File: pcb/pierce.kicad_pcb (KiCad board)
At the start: 2 copper layers, 227.3 x 105.6 mm, 100 parts, among them J1 Conn_01x12, J2 Conn_01x12, J3 Trackpoint, SW1 SW_PUSH, SW10 SW_PUSH, SW11 SW_PUSH, SW12 SW_PUSH, SW13 SW_PUSH, SW14 SW_PUSH, SW15 SW_PUSH, SW16 SW_PUSH, SW17 SW_PUSH, SW18 SW_PUSH, SW19 SW_PUSH, SW2 SW_PUSH, SW20 SW_PUSH, SW21 SW_PUSH, SW22 SW_PUSH, SW23 SW_PUSH, SW24 SW_PUSH, SW25 SW_PUSH, SW26 SW_PUSH, SW27 SW_PUSH, SW28 SW_PUSH, SW29 SW_PUSH, SW3 SW_PUSH, SW30 SW_PUSH, SW31 SW_PUSH, SW32 SW_PUSH, SW33 SW_PUSH, SW34 SW_PUSH, SW35 SW_PUSH, SW36 SW_PUSH, SW37 SW_PUSH, SW38 Rotary_Encoder, SW4 SW_PUSH, SW5 SW_PUSH, SW6 SW_PUSH, SW7 SW_PUSH, SW8 SW_PUSH, SW9 SW_PUSH, U1 Elite-C_reverse

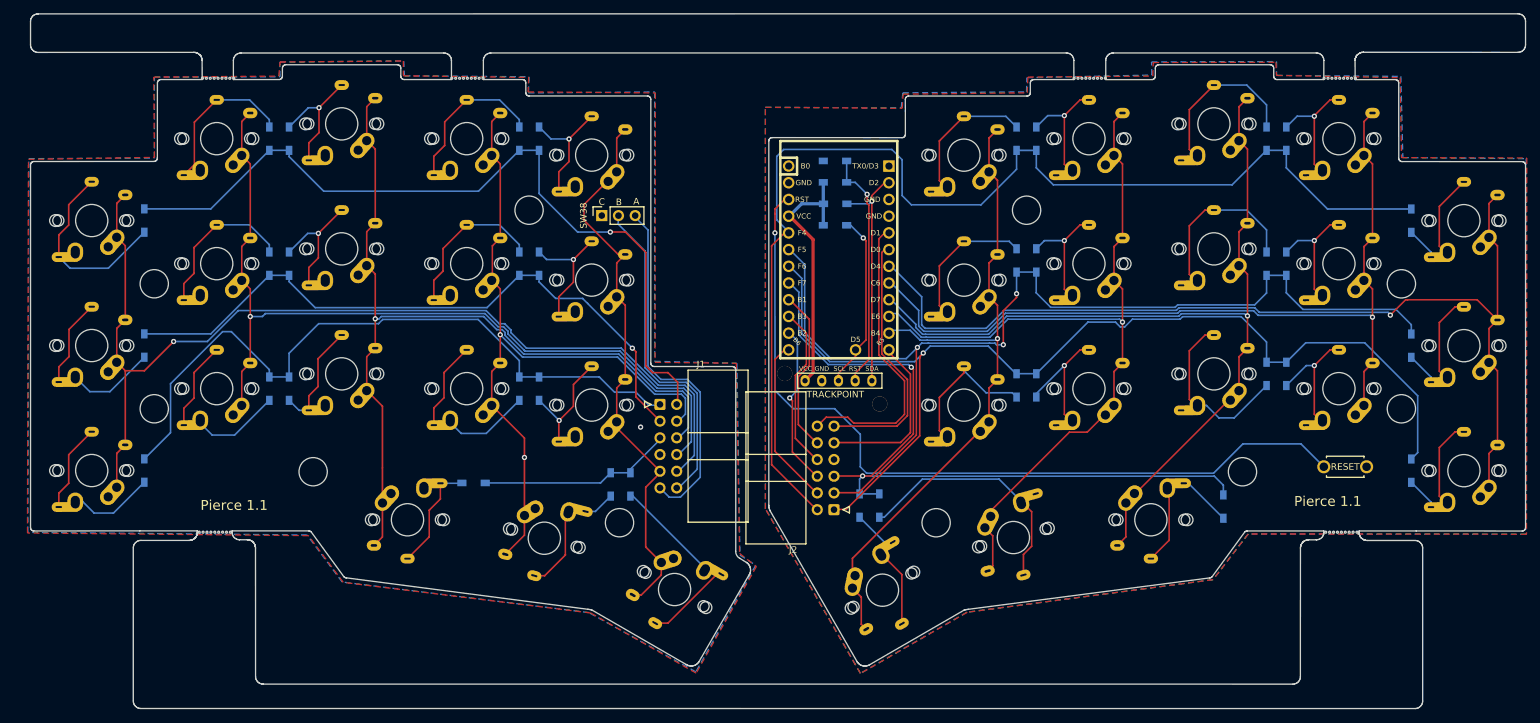
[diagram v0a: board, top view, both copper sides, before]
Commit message: place and route 2.0
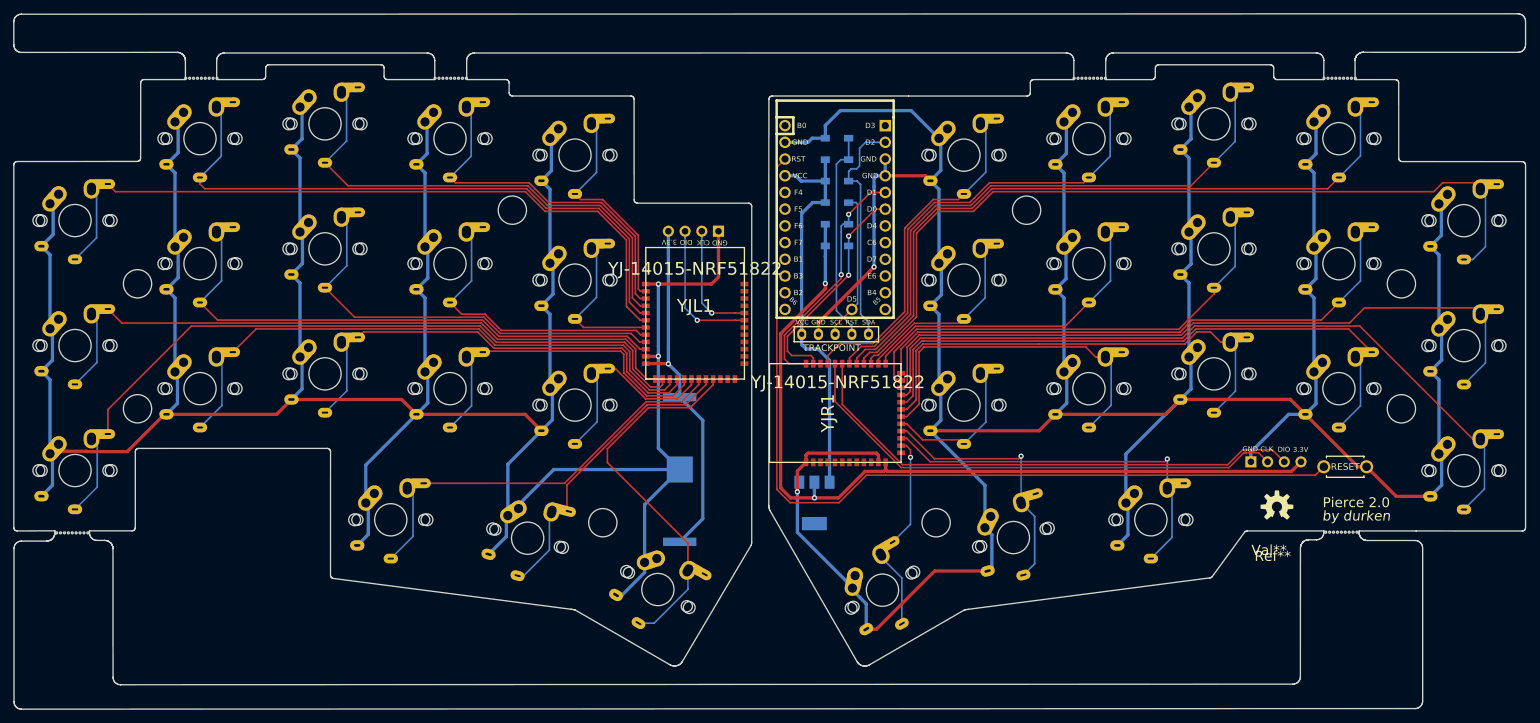
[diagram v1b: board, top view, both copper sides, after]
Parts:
- removed D1, D10, D11, D12, D13, D14, D15, D16, D17, D18, D19, D2, D20, D21, D22, D23, D24, D25, D26, D27, D28, D29, D3, D30, D31, D32, D33, D34, D35, D36, D4, D5, D6, D7, D8, D9: D, kbd:D3_SMD_v2
- removed J1, J2: Conn_01x12, Connector_IDC:IDC-Header_2x06_P2.54mm_Horizontal
- removed J3: Trackpoint, pierce:TRACKPOINT
- removed the REF** at (62.9, 95.0)
- removed the REF** at (101.3, 26.0)
- removed the REF** at (63.4, 26.0)
- removed the Ref** at (53.7, 57.3)
- removed the Ref** at (219.1, 85.8)
- removed the Ref** at (149.5, 70.9)
- removed the Ref** at (162.6, 75.5)
- removed the Ref** at (53.7, 76.3)
- removed the Ref** at (110.6, 46.1)
- removed the Ref** at (124.4, 93.6)
- removed the Ref** at (77.8, 85.8)
- removed SW38: Rotary_Encoder, pierce:Rotary_encoder_conn
- added BT1: Device_Battery_Cell, pierce:BatteryHolder_Keystone_3034_1x20mm, B.Cu at (133.6, 85.5)
- added PROGL1: Conn_01x04_Male, pierce:PinHeader_1x04_P2.54mm_Horizontal, B.Cu at (139.4, 49.3)
- added PROGR1: Conn_01x04_Male, pierce:PinHeader_1x04_P2.54mm_Horizontal, B.Cu at (220.4, 84.3)
- added R4: 4k7, pierce:R_SMD_v2, B.Cu at (157.5, 51.5)
- added R5: 4k7, pierce:R_SMD_v2, B.Cu at (157.5, 48.2)
- added REF**: Breakaway_Tabs, kbd:Breakaway_Tabs, F.Cu at (41.2, 95.1)
- added REF**: Breakaway_Tabs, kbd:Breakaway_Tabs, F.Cu at (98.7, 26.0)
- added REF**: Breakaway_Tabs, kbd:Breakaway_Tabs, F.Cu at (60.8, 26.0)
- added REG1: LD1117S33TR_SOT223, Package_TO_SOT_SMD:SOT-223-3_TabPin2, B.Cu at (154.0, 90.6)
- added Ref**: Val**, pierce:OSHW-LOGO-M, B.Cu at (224.3, 91.2)
- added Ref**: Val**, pierce:OSHW-LOGO-M, F.Cu at (224.3, 91.2)
- added Ref**: Val**, kbd:M2_HOLE_v2, F.Cu at (51.1, 57.3)
- added Ref**: Val**, kbd:M2_HOLE_v2, F.Cu at (51.1, 76.3)
- added Ref**: Val**, kbd:M2_HOLE_v2, F.Cu at (108.1, 46.1)
- added Ref**: Val**, kbd:M2_HOLE_v2, F.Cu at (121.9, 93.6)
- added TP1: Trackpoint, pierce:TRACKPOINT, F.Cu at (152.1, 64.9)
- added YJL1: YJ-14015-NRF51822, pierce:YJ-14015, F.Cu at (135.9, 71.8)
- added YJR1: YJ-14015-NRF51822, pierce:YJ-14015, F.Cu at (167.2, 76.9)
- SW1, SW10, SW11, SW12, SW13, SW14, SW15, SW16, SW17, SW18, SW19, SW2, SW20, SW21, SW22, SW23, SW24, SW25, SW26, SW27, SW28, SW29, SW3, SW30, SW31, SW32, SW33, SW34, SW35, SW36, SW4, SW5, SW6, SW7, SW8, SW9: footprint kbd:keyswitch_cherrymx_alps_choc12_1u -> pierce:keyswitch_cherrymx_alps_choc12_1u
- moved AVR1 6.17 mm to (156.9, 47.2)
- moved R1 3.47 mm to (157.5, 35.1)
- moved C1 3.47 mm to (157.5, 38.4)
- moved R2 3.47 mm to (157.5, 44.9)
- moved R3 3.47 mm to (157.5, 41.7)
- moved SW33 2.54 mm to (130.2, 103.7)
- moved SW15 2.54 mm to (79.6, 33.0), turned to 0 degrees
- moved SW16 2.54 mm to (79.6, 52.0), turned to 0 degrees
- moved SW17 2.54 mm to (79.6, 71.0), turned to 0 degrees
- moved SW18 2.54 mm to (89.6, 93.1)
- moved SW23 2.54 mm to (98.6, 35.2), turned to 0 degrees
- moved SW24 2.54 mm to (98.6, 54.2), turned to 0 degrees
- moved SW25 2.54 mm to (98.6, 73.2), turned to 0 degrees
- moved SW30 2.54 mm to (117.6, 37.7), turned to 0 degrees
- moved SW31 2.54 mm to (117.6, 56.7), turned to 0 degrees
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- renumbered U1 to AVR1, SW37 to RST1
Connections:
- net VCC renamed VCC_R_5V
- AVR1 pad 10: col6 -> Net-(AVR1-Pad10)
- AVR1 pad 11: col5 -> Net-(AVR1-Pad11)
- AVR1 pad 12: col4 -> Net-(AVR1-Pad12)
- AVR1 pad 13: col3 -> Net-(AVR1-Pad13)
- AVR1 pad 14: col2 -> Net-(AVR1-Pad14)
- AVR1 pad 15: col1 -> Net-(AVR1-Pad15)
- AVR1 pad 16: col0 -> Net-(AVR1-Pad16)
- AVR1 pad 17: row3 -> Net-(AVR1-Pad17)
- AVR1 pad 18: row2 -> Net-(AVR1-Pad18)
- AVR1 pad 19: row1 -> Net-(AVR1-Pad19)
- AVR1 pad 20: row0 -> Net-(AVR1-Pad20)
- AVR1 pad 23: GND -> GND_R
- AVR1 pad 3: GND -> GND_R
- AVR1 pad 4: GND -> GND_R
- AVR1 pad 5: rotb -> I2C_SDA
- AVR1 pad 6: rota -> I2C_SCL
- AVR1 pad 7: col9 -> Net-(AVR1-Pad7)
- AVR1 pad 8: col8 -> Net-(AVR1-Pad8)
- AVR1 pad 9: col7 -> Net-(AVR1-Pad9)
- R1 pad 1: GND -> GND_R
- RST1 pad 2: GND -> GND_R
- SW1 pad 1: col0l -> GND_L
- SW1 pad 2: Net-(D1-Pad2) -> SW00L
- SW10 pad 1: col1l -> GND_L
- SW10 pad 2: Net-(D10-Pad2) -> SW21L
- SW11 pad 1: col6 -> GND_R
- SW11 pad 2: Net-(D11-Pad2) -> SW01R
- SW12 pad 1: col6 -> GND_R
- SW12 pad 2: Net-(D12-Pad2) -> SW11R
- SW13 pad 1: col6 -> GND_R
- SW13 pad 2: Net-(D13-Pad2) -> SW21R
- SW14 pad 1: col6 -> GND_R
- SW14 pad 2: Net-(D14-Pad2) -> SW31R
- SW15 pad 1: col2l -> GND_L
- SW15 pad 2: Net-(D15-Pad2) -> SW02L
- SW16 pad 1: col2l -> GND_L
- SW16 pad 2: Net-(D16-Pad2) -> SW12L
- SW17 pad 1: col2l -> GND_L
- SW17 pad 2: Net-(D17-Pad2) -> SW22L
- SW18 pad 1: col2l -> GND_L
- SW18 pad 2: Net-(D18-Pad2) -> SW32L
- SW19 pad 1: col7 -> GND_R
- SW19 pad 2: Net-(D19-Pad2) -> SW02R
- SW2 pad 1: col0l -> GND_L
- SW2 pad 2: Net-(D2-Pad2) -> SW10L
- SW20 pad 1: col7 -> GND_R
- SW20 pad 2: Net-(D20-Pad2) -> SW12R
- SW21 pad 1: col7 -> GND_R
- SW21 pad 2: Net-(D21-Pad2) -> SW22R
- SW22 pad 1: col7 -> GND_R
- SW22 pad 2: Net-(D22-Pad2) -> SW32R
- SW23 pad 1: col3l -> GND_L
- SW23 pad 2: Net-(D23-Pad2) -> SW03L
- SW24 pad 1: col3l -> GND_L
- SW24 pad 2: Net-(D24-Pad2) -> SW13L
- SW25 pad 1: col3l -> GND_L
- SW25 pad 2: Net-(D25-Pad2) -> SW23L
- SW26 pad 1: col3l -> GND_L
- SW26 pad 2: Net-(D26-Pad2) -> SW33L
- SW27 pad 1: col8 -> GND_R
- SW27 pad 2: Net-(D27-Pad2) -> SW03R
- SW28 pad 1: col8 -> GND_R
- SW28 pad 2: Net-(D28-Pad2) -> SW13R
- SW29 pad 1: col8 -> GND_R
- SW29 pad 2: Net-(D29-Pad2) -> SW23R
- SW3 pad 1: col0l -> GND_L
- SW3 pad 2: Net-(D3-Pad2) -> SW20L
- SW30 pad 1: col4l -> GND_L
- SW30 pad 2: Net-(D30-Pad2) -> SW04L
- SW31 pad 1: col4l -> GND_L
- SW31 pad 2: Net-(D31-Pad2) -> SW14L
- SW32 pad 1: col4l -> GND_L
- SW32 pad 2: Net-(D32-Pad2) -> SW24L
- SW33 pad 1: col4l -> GND_L
- SW33 pad 2: Net-(D33-Pad2) -> SW34L
- SW34 pad 1: col9 -> GND_R
- SW34 pad 2: Net-(D34-Pad2) -> SW04R
- SW35 pad 1: col9 -> GND_R
- SW35 pad 2: Net-(D35-Pad2) -> SW14R
- SW36 pad 1: col9 -> GND_R
- SW36 pad 2: Net-(D36-Pad2) -> SW24R
- SW4 pad 1: col5 -> GND_R
- SW4 pad 2: Net-(D4-Pad2) -> SW00R
- SW5 pad 1: col5 -> GND_R
- SW5 pad 2: Net-(D5-Pad2) -> SW10R
- SW6 pad 1: col5 -> GND_R
- SW6 pad 2: Net-(D6-Pad2) -> SW20R
- SW7 pad 1: col5 -> GND_R
- SW7 pad 2: Net-(D7-Pad2) -> SW30R
- SW8 pad 1: col1l -> GND_L
- SW8 pad 2: Net-(D8-Pad2) -> SW01L
- SW9 pad 1: col1l -> GND_L
- SW9 pad 2: Net-(D9-Pad2) -> SW11L
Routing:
- net GND_R: track 0.00 -> 522.9 mm, vias 0 -> 2
- net GND_L: track 0.00 -> 470.2 mm, vias 0 -> 2
- net row0: track 178.6 -> 0.00 mm
- net row2: track 163.2 -> 0.00 mm, vias 1 -> 0
- net row1: track 161.8 -> 0.00 mm, vias 3 -> 0
- net col0l: track 155.7 -> 0.00 mm, vias 1 -> 0
- net col9: track 150.3 -> 0.00 mm, vias 1 -> 0
- net col7: track 137.0 -> 0.00 mm, vias 1 -> 0
- net col2l: track 132.2 -> 0.00 mm, vias 1 -> 0
- net col1l: track 129.7 -> 0.00 mm, vias 1 -> 0
- net VCC_R_3.3V: track 0.00 -> 128.6 mm, vias 0 -> 2
- net SW04R: track 0.00 -> 127.7 mm
- net col8: track 127.0 -> 0.00 mm, vias 1 -> 0
- net row0l: track 122.5 -> 0.00 mm, vias 1 -> 0
- net col6: track 121.2 -> 0.00 mm, vias 1 -> 0
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- removed copper zone on B.Cu, net GND
- removed copper zone on F.Cu, net GND
- removed copper zone on B.Cu, net GND1
- removed copper zone on F.Cu, net GND1
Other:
- board size 227.3 x 105.6 mm -> 229.8 x 105.7 mm
- board text added: "3.3V"
- board text added: "CLK"
- board text added: "DIO"
- board text added: "Pierce 2.0"
- board text added: "by durken"
- board text removed: "A"
- board text removed: "B"
- board text removed: "C"
- board text removed: "COL0"
- board text removed: "COL1"
- board text removed: "COL2"
- board text removed: "COL3"
- board text removed: "COL4"
- board text removed: "COL5"
- board text removed: "COL6"
- board text removed: "COL7"
- board text removed: "COL8"
- board text removed: "Pierce 1.1"
- board text removed: "ROW0"
- board text removed: "ROW1"
- board text removed: "ROW2"
- board text removed: "ROW3"
